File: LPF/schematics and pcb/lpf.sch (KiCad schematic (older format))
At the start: 7 parts, among them P1 BNC, P2 BNC

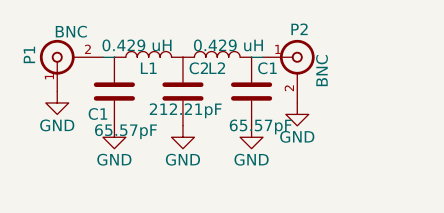
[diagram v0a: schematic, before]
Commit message: asd
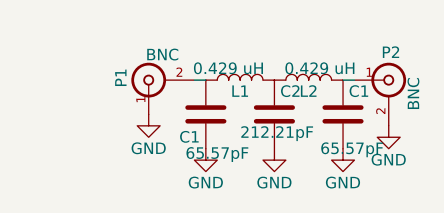
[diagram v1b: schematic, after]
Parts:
- C1, C2: footprint (none) -> Capacitors_SMD:C_0603
- L1, L2: footprint (none) -> Resistors_SMD:R_0603
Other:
- moved on the sheet: C1, C2, L1, L2, P1, P2
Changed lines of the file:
@@
 L C C1
 U 1 1 58C2D76A
-P 3700 3700
-F 0 "C1" H 3725 3800 50  0000 L CNN
-F 1 "65.57pF" H 3650 3900 50  0000 C TNN
-F 2 "" H 3738 3550 50  0000 C CNN
-F 3 "" H 3700 3700 50  0000 C CNN
-	1    3700 3700
+P 4100 3800
+F 0 "C1" H 4125 3900 50  0000 L CNN
+F 1 "65.57pF" H 4050 4000 50  0000 C TNN
+F 2 "Capacitors_SMD:C_0603" H 4138 3650 50  0001 C CNN
+F 3 "" H 4100 3800 50  0000 C CNN
+	1    4100 3800
 	-1   0    0    1
 $EndComp
@@
 L C C2
 U 1 1 58C2D8EA
-P 4000 3700
-F 0 "C2" H 4025 3800 50  0000 L CNN
-F 1 "212.21pF" H 3850 3650 50  0000 L TNN
-F 2 "" H 4038 3550 50  0000 C CNN
-F 3 "" H 4000 3700 50  0000 C CNN
-	1    4000 3700
+P 4400 3800
+F 0 "C2" H 4425 3900 50  0000 L CNN
+F 1 "212.21pF" H 4250 3750 50  0000 L TNN
+F 2 "Capacitors_SMD:C_0603" H 4400 3150 50  0001 C CNN
+F 3 "" H 4400 3800 50  0000 C CNN
+	1    4400 3800
 	1    0    0    -1
 $EndComp
@@
 L L L2
 U 1 1 58C2D90E
-P 4150 3550
-F 0 "L2" V 4100 3550 50  0000 C CNN
-F 1 "0.429 uH" V 4200 3500 50  0000 C CNN
-F 2 "" H 4150 3550 50  0000 C CNN
-F 3 "" H 4150 3550 50  0000 C CNN
-	1    4150 3550
+P 4550 3650
+F 0 "L2" V 4500 3650 50  0000 C CNN
+F 1 "0.429 uH" V 4600 3600 50  0000 C CNN
+F 2 "Resistors_SMD:R_0603" H 4550 3650 50  0001 C CNN
+F 3 "" H 4550 3650 50  0000 C CNN
+	1    4550 3650
 	0    -1   -1   0
 $EndComp
@@
 L C C1
 U 1 1 58C2D93F
-P 4300 3700
-F 0 "C1" H 4325 3800 50  0000 L CNN
-F 1 "65.57pF" H 4200 3550 50  0000 L CNN
-F 2 "" H 4338 3550 50  0000 C CNN
-F 3 "" H 4300 3700 50  0000 C CNN
-	1    4300 3700
+P 4700 3800
+F 0 "C1" H 4725 3900 50  0000 L CNN
+F 1 "65.57pF" H 4600 3650 50  0000 L CNN
+F 2 "Capacitors_SMD:C_0603" H 4738 3650 50  0001 C CNN
+F 3 "" H 4700 3800 50  0000 C CNN
+	1    4700 3800
 	1    0    0    -1
 $EndComp
@@
 L GND #PWR?
 U 1 1 58C2D968
-P 4300 3850
-F 0 "#PWR?" H 4300 3600 50  0001 C CNN
-F 1 "GND" H 4300 3700 50  0000 C CNN
-F 2 "" H 4300 3850 50  0000 C CNN
-F 3 "" H 4300 3850 50  0000 C CNN
-	1    4300 3850
+P 4700 3950
+F 0 "#PWR?" H 4700 3700 50  0001 C CNN
+F 1 "GND" H 4700 3800 50  0000 C CNN
+F 2 "" H 4700 3950 50  0000 C CNN
+F 3 "" H 4700 3950 50  0000 C CNN
+	1    4700 3950
 	1    0    0    -1
 $EndComp
@@
 L GND #PWR?
 U 1 1 58C2D986
-P 3700 3850
-F 0 "#PWR?" H 3700 3600 50  0001 C CNN
-F 1 "GND" H 3700 3700 50  0000 C CNN
-F 2 "" H 3700 3850 50  0000 C CNN
-F 3 "" H 3700 3850 50  0000 C CNN
-	1    3700 3850
+P 4100 3950
+F 0 "#PWR?" H 4100 3700 50  0001 C CNN
+F 1 "GND" H 4100 3800 50  0000 C CNN
+F 2 "" H 4100 3950 50  0000 C CNN
+F 3 "" H 4100 3950 50  0000 C CNN
+	1    4100 3950
 	1    0    0    -1
 $EndComp
@@
 L GND #PWR?
 U 1 1 58C2D9A4
-P 4000 3850
-F 0 "#PWR?" H 4000 3600 50  0001 C CNN
-F 1 "GND" H 4000 3700 50  0000 C CNN
-F 2 "" H 4000 3850 50  0000 C CNN
-F 3 "" H 4000 3850 50  0000 C CNN
-	1    4000 3850
+P 4400 3950
+F 0 "#PWR?" H 4400 3700 50  0001 C CNN
+F 1 "GND" H 4400 3800 50  0000 C CNN
+F 2 "" H 4400 3950 50  0000 C CNN
+F 3 "" H 4400 3950 50  0000 C CNN
+	1    4400 3950
 	1    0    0    -1
 $EndComp
@@
 L BNC P2
 U 1 1 58C2D9CC
-P 4500 3550
-F 0 "P2" H 4510 3670 50  0000 C CNN
-F 1 "BNC" V 4610 3490 50  0000 C CNN
-F 2 "" H 4500 3550 50  0000 C CNN
-F 3 "" H 4500 3550 50  0000 C CNN
-	1    4500 3550
+P 4900 3650
+F 0 "P2" H 4910 3770 50  0000 C CNN
+F 1 "BNC" V 5010 3590 50  0000 C CNN
+F 2 "" H 4900 3650 50  0000 C CNN
+F 3 "" H 4900 3650 50  0000 C CNN
+	1    4900 3650
 	1    0    0    -1
 $EndComp
 Wire Wire Line
-	4350 3550 4300 3550
+	4750 3650 4700 3650
 Wire Wire Line
-	3700 3550 3650 3550
+	4100 3650 4050 3650
 $Comp
 L BNC P1
 U 1 1 58C2E002
-P 3450 3550
-F 0 "P1" H 3460 3670 50  0000 C CNN
-F 1 "BNC" V 3560 3490 50  0000 C CNN
-F 2 "" H 3450 3550 50  0000 C CNN
-F 3 "" H 3450 3550 50  0000 C CNN
-	1    3450 3550
+P 3850 3650
+F 0 "P1" H 3860 3770 50  0000 C CNN
+F 1 "BNC" V 3960 3590 50  0000 C CNN
+F 2 "" H 3850 3650 50  0000 C CNN
+F 3 "" H 3850 3650 50  0000 C CNN
+	1    3850 3650
 	0    -1   -1   0
 $EndComp
@@
 L GND #PWR?
 U 1 1 58C2E15B
-P 3450 3700
-F 0 "#PWR?" H 3450 3450 50  0001 C CNN
-F 1 "GND" H 3450 3550 50  0000 C CNN
-F 2 "" H 3450 3700 50  0000 C CNN
-F 3 "" H 3450 3700 50  0000 C CNN
-	1    3450 3700
+P 3850 3800
+F 0 "#PWR?" H 3850 3550 50  0001 C CNN
+F 1 "GND" H 3850 3650 50  0000 C CNN
+F 2 "" H 3850 3800 50  0000 C CNN
+F 3 "" H 3850 3800 50  0000 C CNN
+	1    3850 3800
 	1    0    0    -1
 $EndComp
@@
 L GND #PWR?
 U 1 1 58C2E17D
-P 4500 3750
-F 0 "#PWR?" H 4500 3500 50  0001 C CNN
-F 1 "GND" H 4500 3600 50  0000 C CNN
-F 2 "" H 4500 3750 50  0000 C CNN
-F 3 "" H 4500 3750 50  0000 C CNN
-	1    4500 3750
+P 4900 3850
+F 0 "#PWR?" H 4900 3600 50  0001 C CNN
+F 1 "GND" H 4900 3700 50  0000 C CNN
+F 2 "" H 4900 3850 50  0000 C CNN
+F 3 "" H 4900 3850 50  0000 C CNN
+	1    4900 3850
 	1    0    0    -1
 $EndComp
@@
 L L L1
 U 1 1 58C2D886
-P 3850 3550
-F 0 "L1" V 3800 3550 50  0000 C CNN
-F 1 "0.429 uH" V 3900 3600 50  0000 C CNN
-F 2 "" H 3850 3550 50  0000 C CNN
-F 3 "" H 3850 3550 50  0000 C CNN
-	1    3850 3550
+P 4250 3650
+F 0 "L1" V 4200 3650 50  0000 C CNN
+F 1 "0.429 uH" V 4300 3700 50  0000 C CNN
+F 2 "Resistors_SMD:R_0603" H 4250 3650 50  0001 C CNN
+F 3 "" H 4250 3650 50  0000 C CNN
+	1    4250 3650
 	0    -1   -1   0
 $EndComp

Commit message: asdf
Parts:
- P1, P2: footprint (none) -> Connectors_Molex:Molex_SMA_Jack_Edge_Mount
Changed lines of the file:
@@
 F 0 "P2" H 4910 3770 50  0000 C CNN
 F 1 "BNC" V 5010 3590 50  0000 C CNN
-F 2 "" H 4900 3650 50  0000 C CNN
+F 2 "Connectors_Molex:Molex_SMA_Jack_Edge_Mount" H 4900 3650 50  0001 C CNN
 F 3 "" H 4900 3650 50  0000 C CNN
 	1    4900 3650
@@
 F 0 "P1" H 3860 3770 50  0000 C CNN
 F 1 "BNC" V 3960 3590 50  0000 C CNN
-F 2 "" H 3850 3650 50  0000 C CNN
+F 2 "Connectors_Molex:Molex_SMA_Jack_Edge_Mount" H 3850 3650 50  0001 C CNN
 F 3 "" H 3850 3650 50  0000 C CNN
 	1    3850 3650
